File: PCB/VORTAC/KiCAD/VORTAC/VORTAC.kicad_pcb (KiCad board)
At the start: 4 copper layers, 46 x 52.4 mm, 128 parts, among them IC1 TMC2209-LA, J1 DEBUG, J10 FAN_01_V, J11 FAN_02_V, J12 LED_V, J13 THERM_R, J14 918-418K2023S40001, J15 STEPPER, J16 IO, J2 Molex Micro Fit 3.0, J3 MillMax_004, J4 MillMax_004, J5 USB_HOST, J6 HOTEND, J7 FAN_01, J8 FAN_02, J9 LED, Q1 Q_PMOS_GSD, Q2 Q_NMOS_GSD, Q3 WSD4066DN, Q4 Q_NMOS_GSD, Q5 WSD4066DN, Q6 Q_PNP_BEC, Q7 Q_NPN_BEC, U1 TLV73333PDBV, U2 STM32F103C8Tx, U3 TPS54335ADRCR, U4 TPS54335ADRCR, U5 ADXL345BCCZ-RL7, U6 TJA1040T

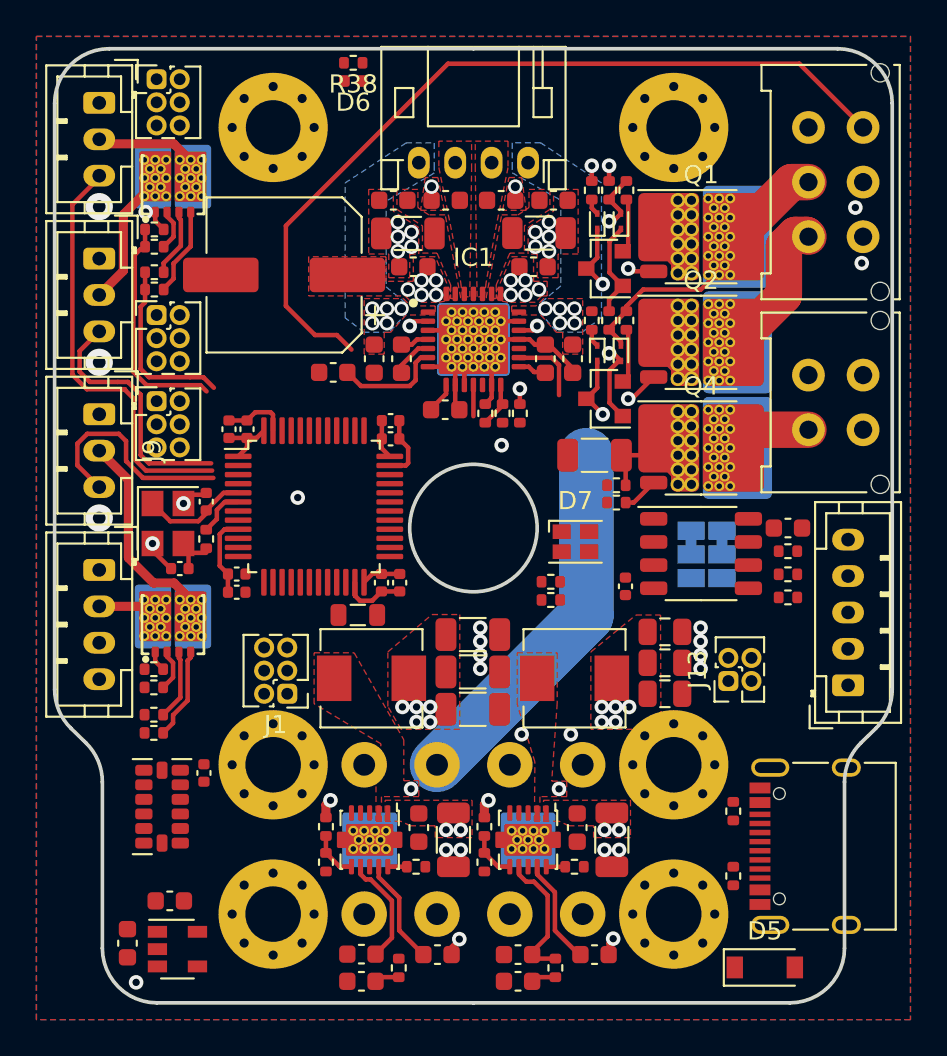
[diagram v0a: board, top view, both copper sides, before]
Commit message: Holiday Break <3
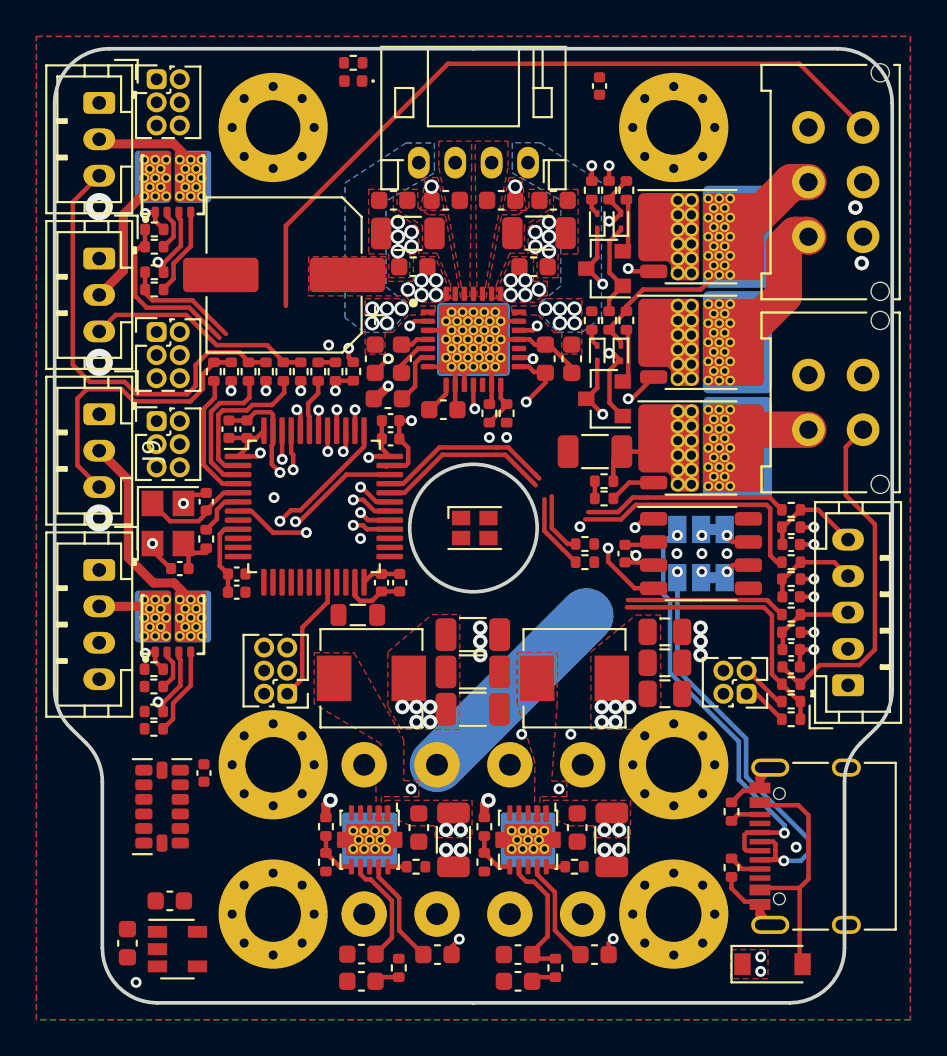
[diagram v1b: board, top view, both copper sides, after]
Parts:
- added C46: 0.1uF 16V, Capacitor_SMD:C_0402_1005Metric, F.Cu at (117.5, 100.9)
- added C47: 0.1uF 16V, Capacitor_SMD:C_0402_1005Metric, F.Cu at (117.5, 103.8)
- added C48: 0.1uF 16V, Capacitor_SMD:C_0402_1005Metric, F.Cu at (117.5, 106.7)
- added C49: 0.1uF 16V, Capacitor_SMD:C_0402_1005Metric, F.Cu at (106.9, 75.7)
- added R39: 10K, Resistor_SMD:R_0402_1005Metric, F.Cu at (87.7, 91.4)
- added R40: 10K, Resistor_SMD:R_0402_1005Metric, F.Cu at (89.6, 91.4)
- added R41: 10K, Resistor_SMD:R_0402_1005Metric, F.Cu at (85.7, 91.4)
- added R42: 10K, Resistor_SMD:R_0402_1005Metric, F.Cu at (117.5, 99.0)
- added R43: 10K, Resistor_SMD:R_0402_1005Metric, F.Cu at (117.5, 101.9)
- added R44: 10K, Resistor_SMD:R_0402_1005Metric, F.Cu at (117.5, 104.8)
- added R45: 10K, Resistor_SMD:R_0402_1005Metric, F.Cu at (88.6, 91.4)
- added R46: 10K, Resistor_SMD:R_0402_1005Metric, F.Cu at (90.5, 91.4)
- added R47: 10K, Resistor_SMD:R_0402_1005Metric, F.Cu at (86.7, 91.4)
- added R48: 10K, Resistor_SMD:R_0402_1005Metric, F.Cu at (117.5, 100.0)
- added R49: 10K, Resistor_SMD:R_0402_1005Metric, F.Cu at (117.5, 102.8)
- added R50: 10K, Resistor_SMD:R_0402_1005Metric, F.Cu at (117.5, 105.7)
- added R51: 10K, Resistor_SMD:R_0402_1005Metric, F.Cu at (91.5, 91.4)
- added R52: 10K, Resistor_SMD:R_0402_1005Metric, F.Cu at (92.4, 91.4)
- C2: footprint Capacitor_SMD:C_0603_1608Metric -> Capacitor_SMD:C_0402_1005Metric
- moved R32 9.43 mm to (93.4, 91.4)
- moved C2 7.63 mm to (117.5, 107.6)
- moved R21 7.31 mm to (117.5, 108.6), turned to 180 degrees
- moved R2 6.99 mm to (117.5, 109.5)
- moved R1 6.69 mm to (117.5, 110.5)
- moved D7 5.58 mm to (100.1, 100.0)
- moved C24 3.33 mm to (95.3, 92.9)
- moved R35 2.80 mm to (106.1, 101.9)
- moved R36 2.80 mm to (106.1, 100.9)
- moved C35 1.80 mm to (108.3, 101.4)
- moved JP1 1.79 mm to (112.5, 100.1), turned to 180 degrees
- moved JP2 1.39 mm to (112.5, 102.7), turned to 180 degrees
- moved J13 1.22 mm to (115.0, 109.1), turned to 180 degrees
- moved J12 1.09 mm to (82.6, 94.1)
- moved J11 0.93 mm to (82.6, 89.2)
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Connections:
- U2 pad 2: Net-(U2-Pad2) -> FAN_2_TACHO_PIN
- U2 pad 20: Net-(U2-Pad20) -> BOOT_1
- U2 pad 26: Net-(U2-Pad26) -> IO_3_OUT
- U2 pad 27: Net-(U2-Pad27) -> IO_2_OUT
- U2 pad 28: Net-(U2-Pad28) -> IO_1_OUT
- U2 pad 29: Net-(U2-Pad29) -> HEATER_GATE
- U2 pad 3: Net-(U2-Pad3) -> FAN_1_TACHO_PIN
- U2 pad 30: Net-(U2-Pad30) -> TMC_UART_TX
- U2 pad 31: Net-(U2-Pad31) -> TMC_UART_RX
- U2 pad 38: Net-(U2-Pad38) -> TMC_DIR
- U2 pad 39: Net-(U2-Pad39) -> TMC_DIAG
- U2 pad 4: Net-(U2-Pad4) -> LED_1_PWM_PIN
- U2 pad 40: Net-(U2-Pad40) -> TMC_ENN
- U2 pad 41: Net-(U2-Pad41) -> TMC_STEP
- U2 pad 42: Net-(U2-Pad42) -> LED_0
- U2 pad 43: Net-(U2-Pad43) -> TOOL_ID_PIN
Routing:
- net CAN_RX: track 0.00 -> 29.1 mm, vias 0 -> 2
- net CAN_TX: track 0.00 -> 26.0 mm, vias 0 -> 2
- net USB_D-: track 0.00 -> 23.5 mm, vias 0 -> 2
- net USB_D+: track 0.00 -> 23.5 mm, vias 0 -> 2
- net GND: track 51.7 -> 71.2 mm, vias 30 -> 41
- net THERM_1_OUT: track 0.00 -> 19.4 mm
- net +3.3VA: track 4.50 -> 23.6 mm
- net HEATER_GATE: track 0.00 -> 16.1 mm, vias 0 -> 1
- net THERM_1_PIN: track 0.00 -> 14.5 mm
- net DEBUG_SWCLK: track 0.00 -> 14.5 mm, vias 0 -> 1
- net TMC_DIR: track 1.10 -> 15.4 mm
- net IO_2_OUT_PIN: track 0.00 -> 13.9 mm
- net Net-(R35-Pad2): track 0.00 -> 13.7 mm
- net Net-(D5-Pad2): track 0.00 -> 13.5 mm
- net DEBUG_SWDIO: track 0.00 -> 13.4 mm, vias 0 -> 1
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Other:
- net class Default: via_dia 0.8 -> 0.6; via_drill 0.4 -> 0.3
